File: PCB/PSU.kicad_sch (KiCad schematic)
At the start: 77 parts, among them U1 AMS1117-3.3, U6 AP2127K-ADJ

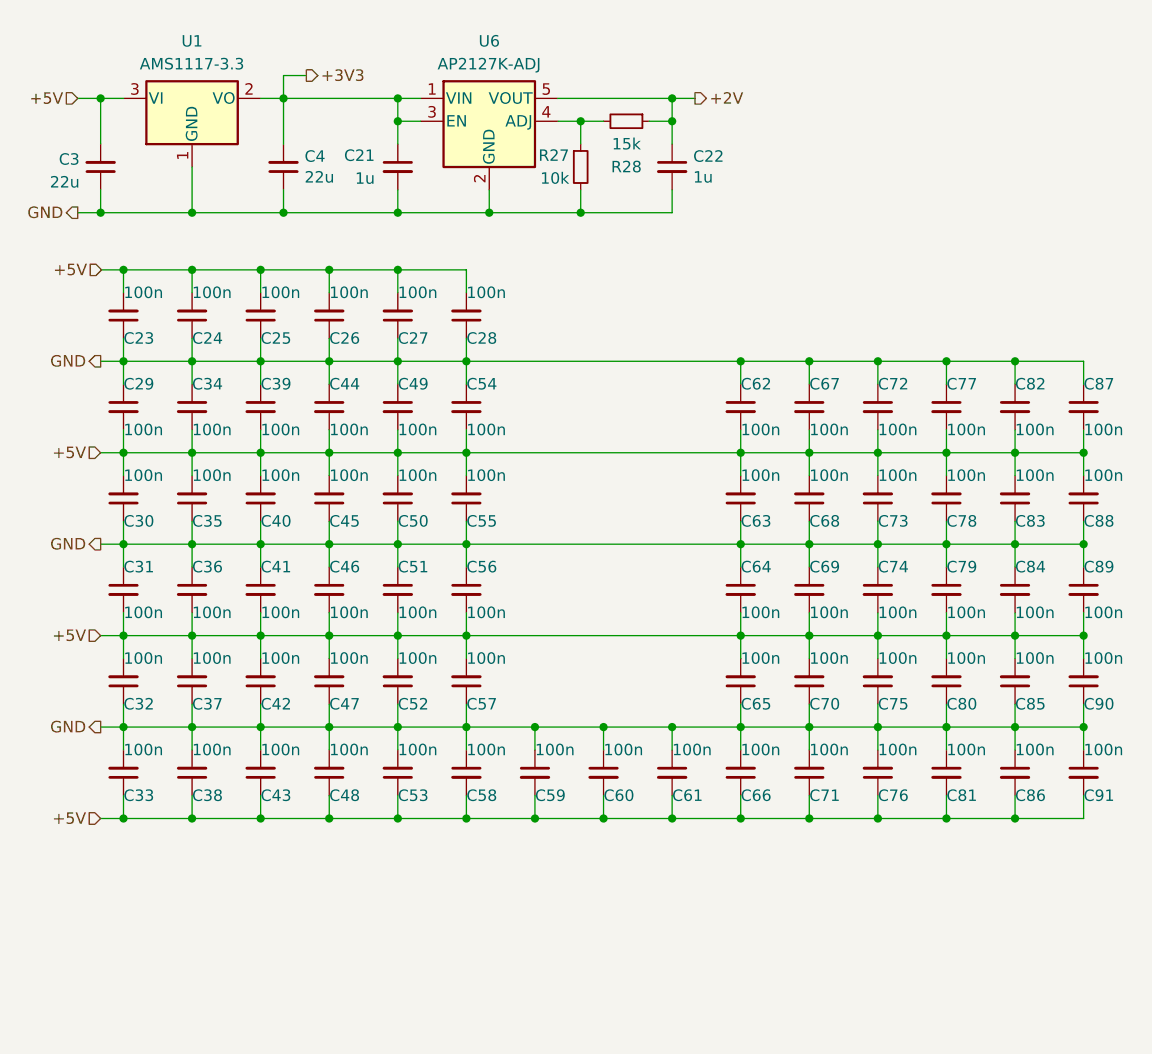
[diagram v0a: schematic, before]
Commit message: Massive mistake corrections and clarifications.
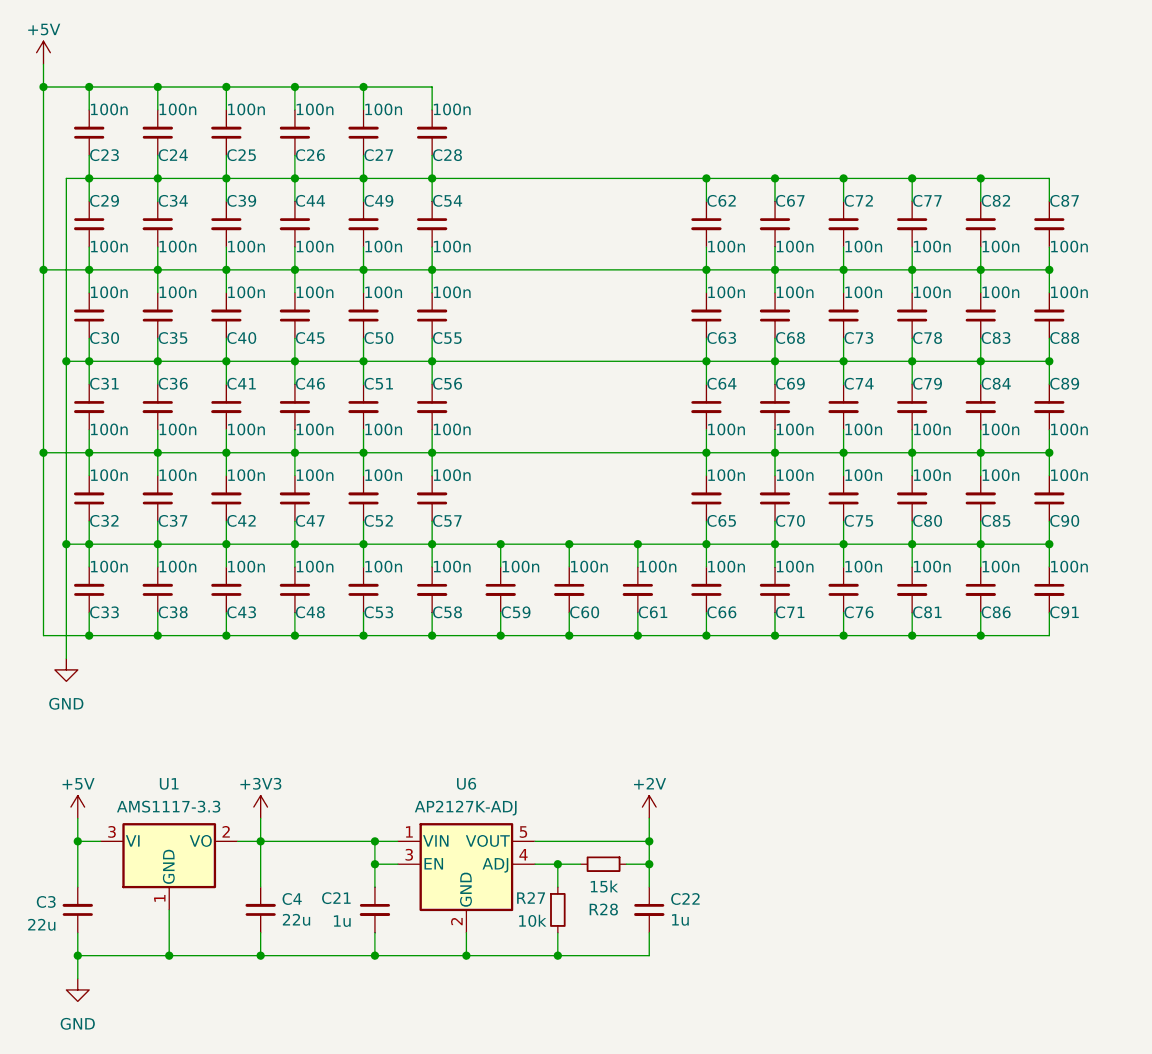
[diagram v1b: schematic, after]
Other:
- moved on the sheet: C21, C22, C23, C24, C25, C26, C27, C28, C29, C3, C30, C31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

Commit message: Rewording of readme. Added files for JLC PCBA. Changed USB C connector and moved it away from board.
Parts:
- C21, C22: LCSC (none) -> C15849; LCSC part number C15849 -> (none)
- C23, C24, C25, C26, C27, C28, C29, C30, C31, C32, C33, C34, C35, C36, C37, C38, C39, C40, C41, C42, C43, C44, C45, C46, C47, C48, C49, C50, C51, C52, C53, C54, C55, C56, C57, C58, C59, C60, C61, C62, C63, C64, C65, C66, C67, C68, C69, C70, C71, C72, C73, C74, C75, C76, C77, C78, C79, C80, C81, C82, C83, C84, C85, C86, C87, C88, C89, C90, C91: LCSC (none) -> C1525; LCSC part number C1525 -> (none)
- C3, C4: LCSC (none) -> C45783; LCSC part number C45783 -> (none)
- R27: LCSC (none) -> C25744; LCSC part number C25744 -> (none)
- R28: LCSC (none) -> C25756; LCSC part number C25756 -> (none)
- U1: LCSC (none) -> C6186; LCSC part number C6186 -> (none)
- U6: LCSC (none) -> C96343; LCSC part number C96343 -> (none)

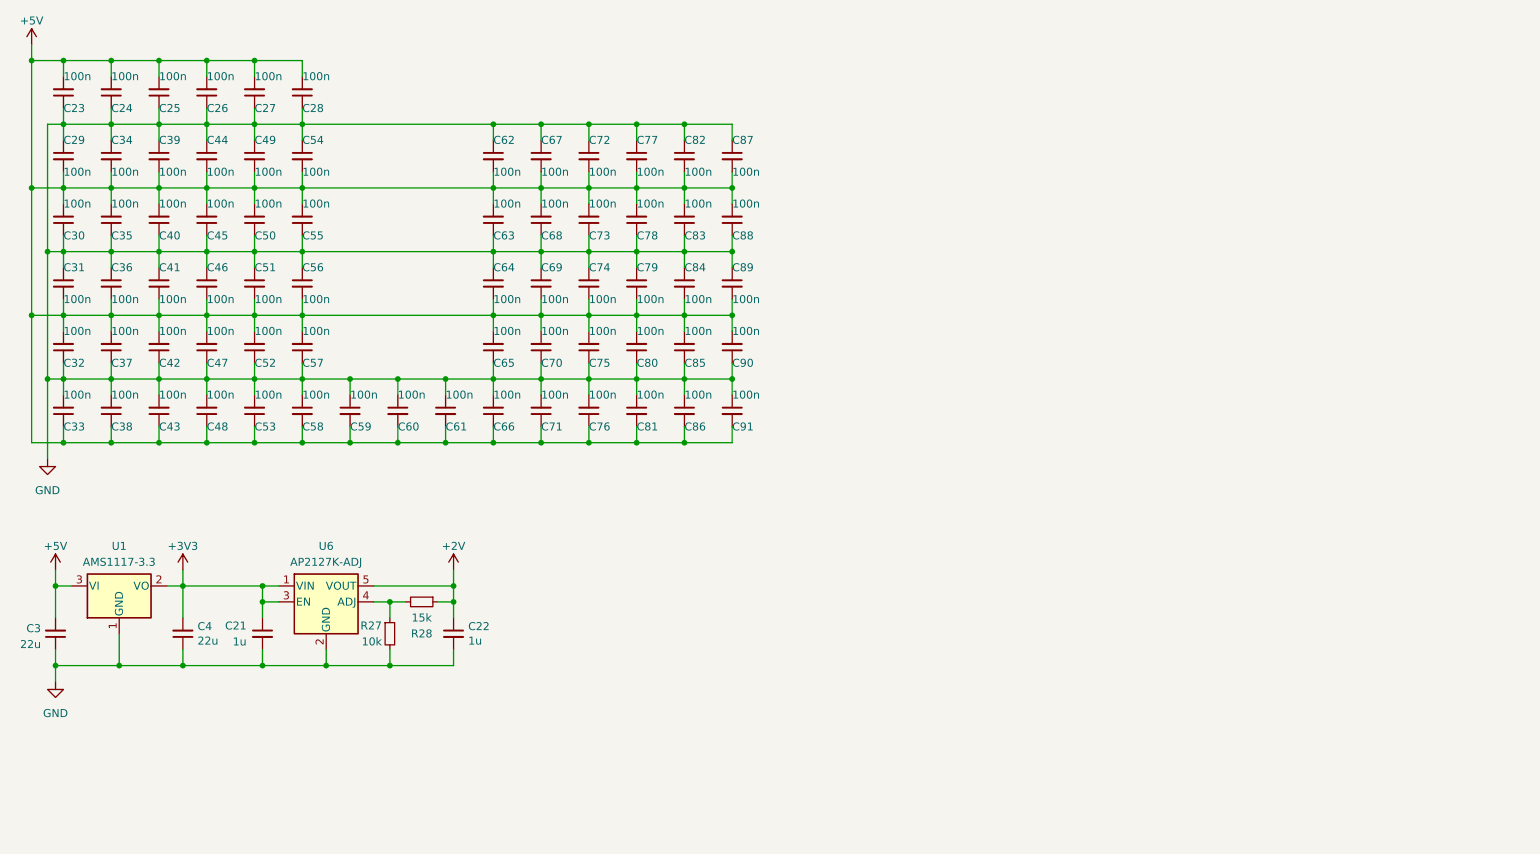
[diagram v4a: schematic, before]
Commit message: Initial V2.0 update.
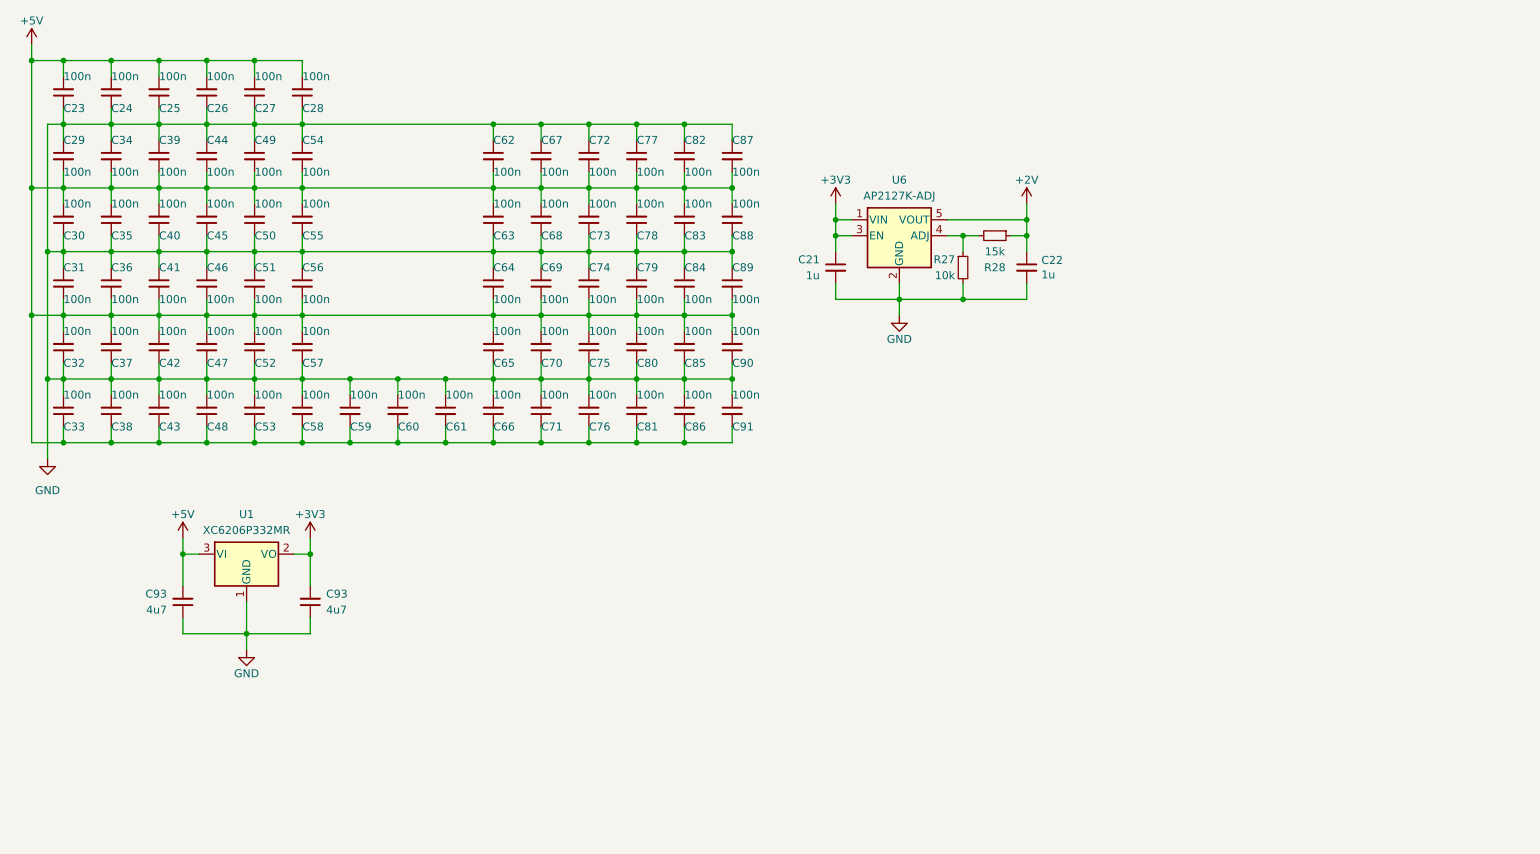
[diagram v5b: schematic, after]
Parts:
- removed C3, C4: 22u, Capacitor_SMD:C_0805_2012Metric, symbol Device:C_Small
- removed U1: AMS1117-3.3, Package_TO_SOT_SMD:SOT-223-3_TabPin2, symbol Regulator_Linear:AMS1117-3.3
- added C93 (x2): 4u7, Capacitor_SMD:C_0603_1608Metric, symbol Device:C_Small
- added U1: XC6206P332MR, Package_TO_SOT_SMD:SOT-23, symbol Regulator_Linear:XC6206PxxxMR
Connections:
- net +3V3: now also C93.2, U1.2 (VO)
- net +5V: now also C93.2, U1.3 (VI)
- net GND: now also C93.1, C93.1, U1.1 (GND)
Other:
- moved on the sheet: C21, C22, R27, R28, U6

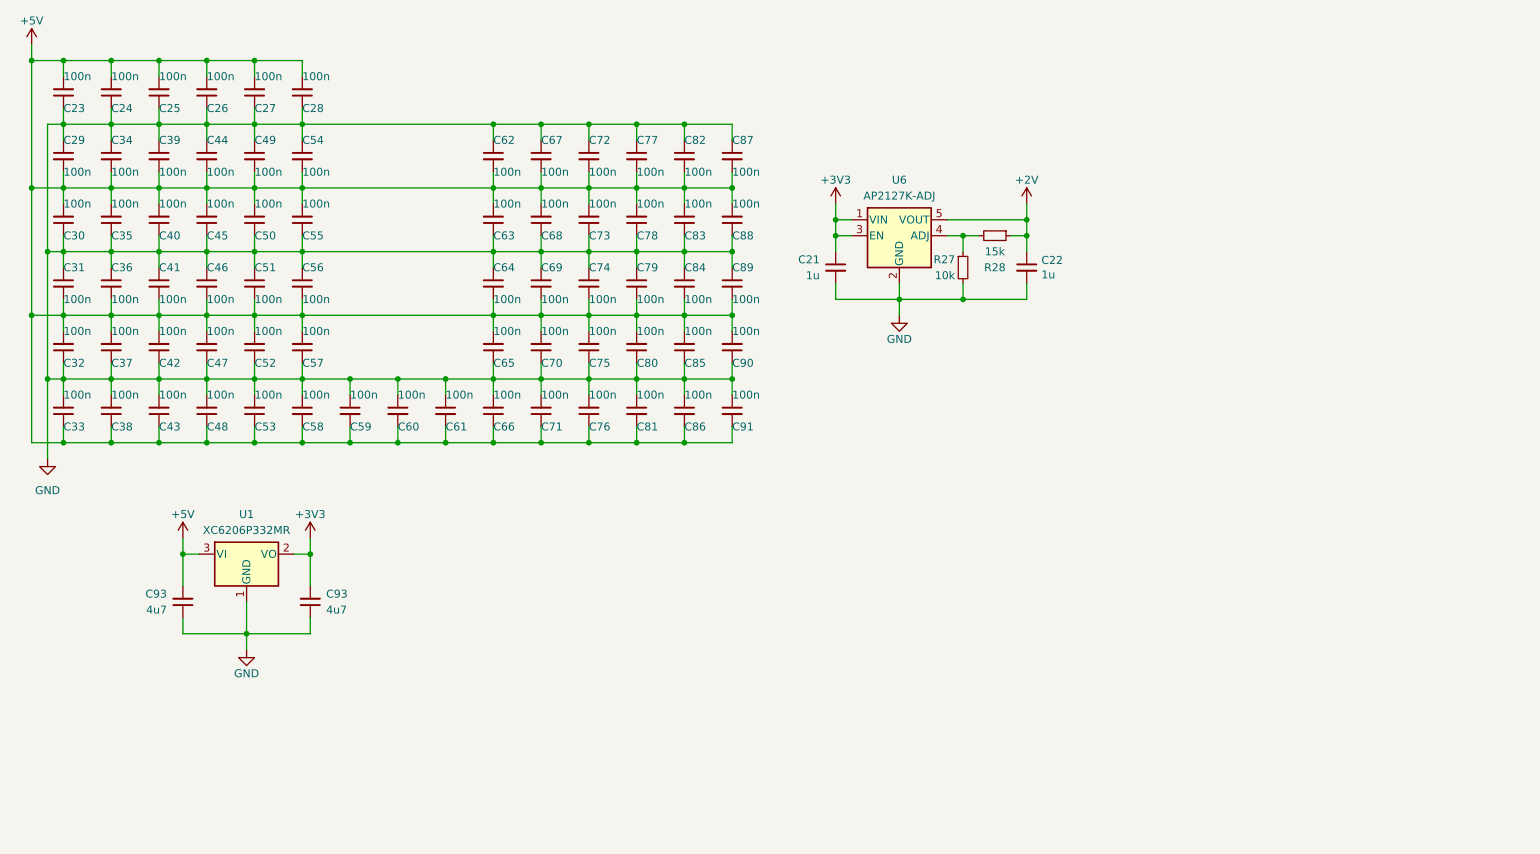
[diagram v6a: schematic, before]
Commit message: Large update.
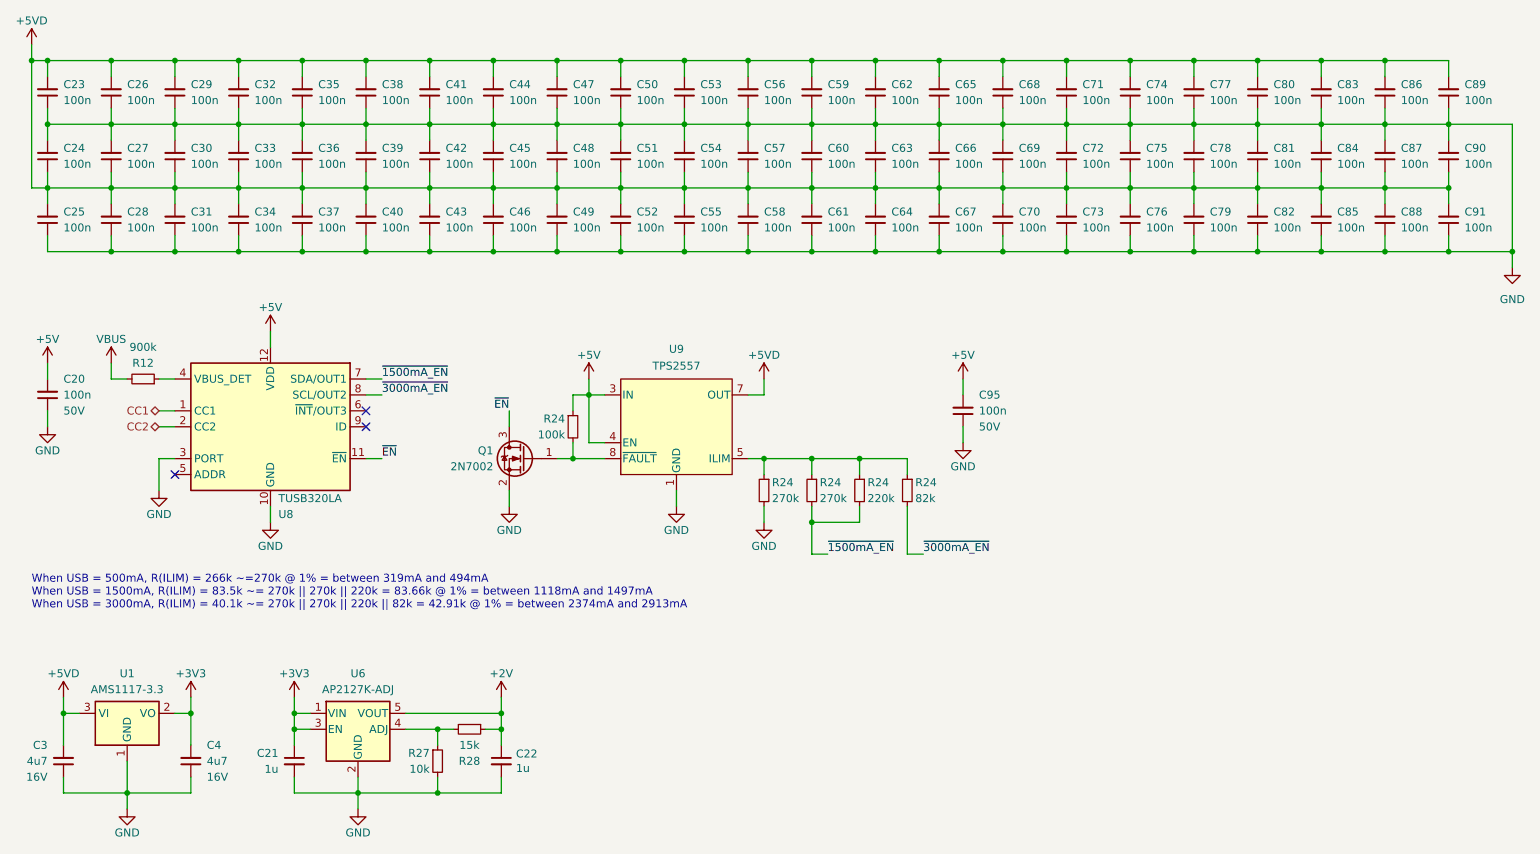
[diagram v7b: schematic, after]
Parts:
- removed C93: 4u7, Capacitor_SMD:C_0603_1608Metric, symbol Device:C_Small
- removed U1: XC6206P332MR, Package_TO_SOT_SMD:SOT-23, symbol Regulator_Linear:XC6206PxxxMR
- added C20, C95: 100n, Capacitor_SMD:C_0402_1005Metric, symbol Device:C_Small
- added C4: 4u7, Capacitor_SMD:C_0603_1608Metric, symbol Device:C_Small
- added Q1: 2N7002, Package_TO_SOT_SMD:SOT-23, symbol Transistor_FET:2N7002
- added R12: 900k, Resistor_SMD:R_0402_1005Metric, symbol Device:R_Small
- added R24 (x2): 270k, Resistor_SMD:R_0402_1005Metric, symbol Device:R_Small
- added R24: 82k, Resistor_SMD:R_0402_1005Metric, symbol Device:R_Small
- added R24: 220k, Resistor_SMD:R_0402_1005Metric, symbol Device:R_Small
- added R24: 100k, Resistor_SMD:R_0402_1005Metric, symbol Device:R_Small
- added U1: AMS1117-3.3, Package_TO_SOT_SMD:SOT-223-3_TabPin2, symbol Regulator_Linear:AMS1117-3.3
- added U8: TUSB320LA, Honeydew:Texas_X2QFN-12_1.6x1.6mm_P0.4mm, symbol Interface_USB:TUSB320I
- added U9: TPS2557, Honeydew:HVSON-8-1EP_3x3mm_P0.65mm_EP1.6x2.4mm, symbol Honeydew:TPS2557
- C21, C22: Voltage (none) -> 50V
- C23, C24, C25, C26, C27, C28, C29, C30, C31, C32, C33, C34, C35, C36, C37, C38, C39, C40, C41, C42, C43, C44, C45, C46, C47, C48, C49, C50, C51, C52, C53, C54, C55, C56, C57, C58, C59, C60, C61, C62, C63, C64, C65, C66, C67, C68, C69, C70, C71, C72, C73, C74, C75, C76, C77, C78, C79, C80, C81, C82, C83, C84, C85, C86, C87, C88, C89, C90, C91: LCSC C1525 -> C307331; Voltage (none) -> 50V
- C3: renamed from C93; Voltage (none) -> 16V
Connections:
- net +3V3: now also C4.2, U1.2 (VO)
- net +5V: now also C20.2, C95.2, R24.1, U8.12 (VDD), U9.2 (IN), U9.3 (IN), U9.4 (EN); no longer C23.2, C24.2, C25.2, C26.2, C27.2, C28.2, C29.2, C3.2, C30.2, C31.2, C32.2, C33.1, C34.2, C35.2, C36.2, C37.2, C38.1, C39.2, C40.2, C41.2, C42.2, C43.1, C44.2, C45.2, C46.2, C47.2, C48.1, C49.2, C50.2, C51.2, C52.2, C53.1, C54.2, C55.2, C56.2, C57.2, C58.2, C59.2, C60.2, C61.2, C62.2, C63.2, C64.2, C65.2, C66.1, C67.2, C68.2, C69.2, C70.2, C71.1, C72.2, C73.2, C74.2, C75.2, C76.1, C77.2, C78.2, C79.2, C80.2, C81.2, C82.2, C83.2, C84.2, C85.2, C86.2, C87.2, C88.2, C89.2, C90.2, C91.2
- net GND: now also C24.2, C27.2, C30.2, C36.2, C38.1, C39.2, C42.2, C43.1, C45.2, C51.2, C53.1, C54.2, C57.2, C60.2, C63.2, C69.2, C71.1, C72.2, C75.2, C76.1, C78.2, C81.2, C84.2, C87.2, C90.2, C20.1, C4.1, C95.1, Q1.2 (S), R24.2, U1.1 (GND), U8.10 (GND), U8.3 (PORT), U9.1 (GND), U9.9 (GND); no longer C24.1, C27.1, C30.1, C36.1, C38.2, C39.1, C42.1, C43.2, C45.1, C51.1, C53.2, C54.1, C57.1, C60.1, C63.1, C69.1, C71.2, C72.1, C75.1, C76.2, C78.1, C81.1, C84.1, C87.1, C90.1
- new net: R24.1, R24.1, R24.1, R24.1, U9.5 (ILIM)
- new net: Q1.1 (G), R24.2, U9.8 (~{FAULT})
- new net: R12.1, U8.4 (VBUS_DET)
- new net +5VD: C23.2, C24.1, C25.2, C26.2, C27.1, C28.2, C29.2, C3.2, C30.1, C31.2, C32.2, C33.1, C34.2, C35.2, C36.1, C37.2, C38.2, C39.1, C40.2, C41.2, C42.1, C43.2, C44.2, C45.1, C46.2, C47.2, C48.1, C49.2, C50.2, C51.1, C52.2, C53.2, C54.1, C55.2, C56.2, C57.1, C58.2, C59.2, C60.1, C61.2, C62.2, C63.1, C64.2, C65.2, C66.1, C67.2, C68.2, C69.1, C70.2, C71.2, C72.1, C73.2, C74.2, C75.1, C76.2, C77.2, C78.1, C79.2, C80.2, C81.1, C82.2, C83.2, C84.1, C85.2, C86.2, C87.1, C88.2, C89.2, C90.1, C91.2, U1.3 (VI), U9.6 (OUT), U9.7 (OUT)
- new net CC1: U8.1 (CC1)
- new net CC2: U8.2 (CC2)
- new net VBUS: R12.2
- new net ~{1500mA_EN}: R24.2, R24.2, U8.7 (SDA/OUT1)
- new net ~{3000mA_EN}: R24.2, U8.8 (SCL/OUT2)
- new net ~{EN}: Q1.3 (D), U8.11 (~{EN})
- no-connect marks 0 -> 3
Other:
- note added: "When USB = 500mA, R(ILIM) = 266k ~=270k @ 1% = between 319mA and 494mA When USB = 1500mA, R(ILIM) = 83.5k ~= 270k || 270k || 220k = 83.66k @ 1% = between 1118mA and 1497mA When USB = 3000mA, R(ILIM) = 40.1k ~= 270k || 270k || 220k || 82k = 42.91k @ 1% = between 2374mA and 2913mA"
- moved on the sheet: C21, C22, C3, R27, R28, U6
